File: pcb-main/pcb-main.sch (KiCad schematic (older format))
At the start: 26 parts, among them J1 AVR-ISP-6, J2 Conn_02x06_Counter_Clockwise, J3 Conn_02x02_Counter_Clockwise, M1 Stepper_Motor, U1 ATmega328P-AU, U2 HT1621B, U3 VIM878, U4 TLSM, Y1 Crystal

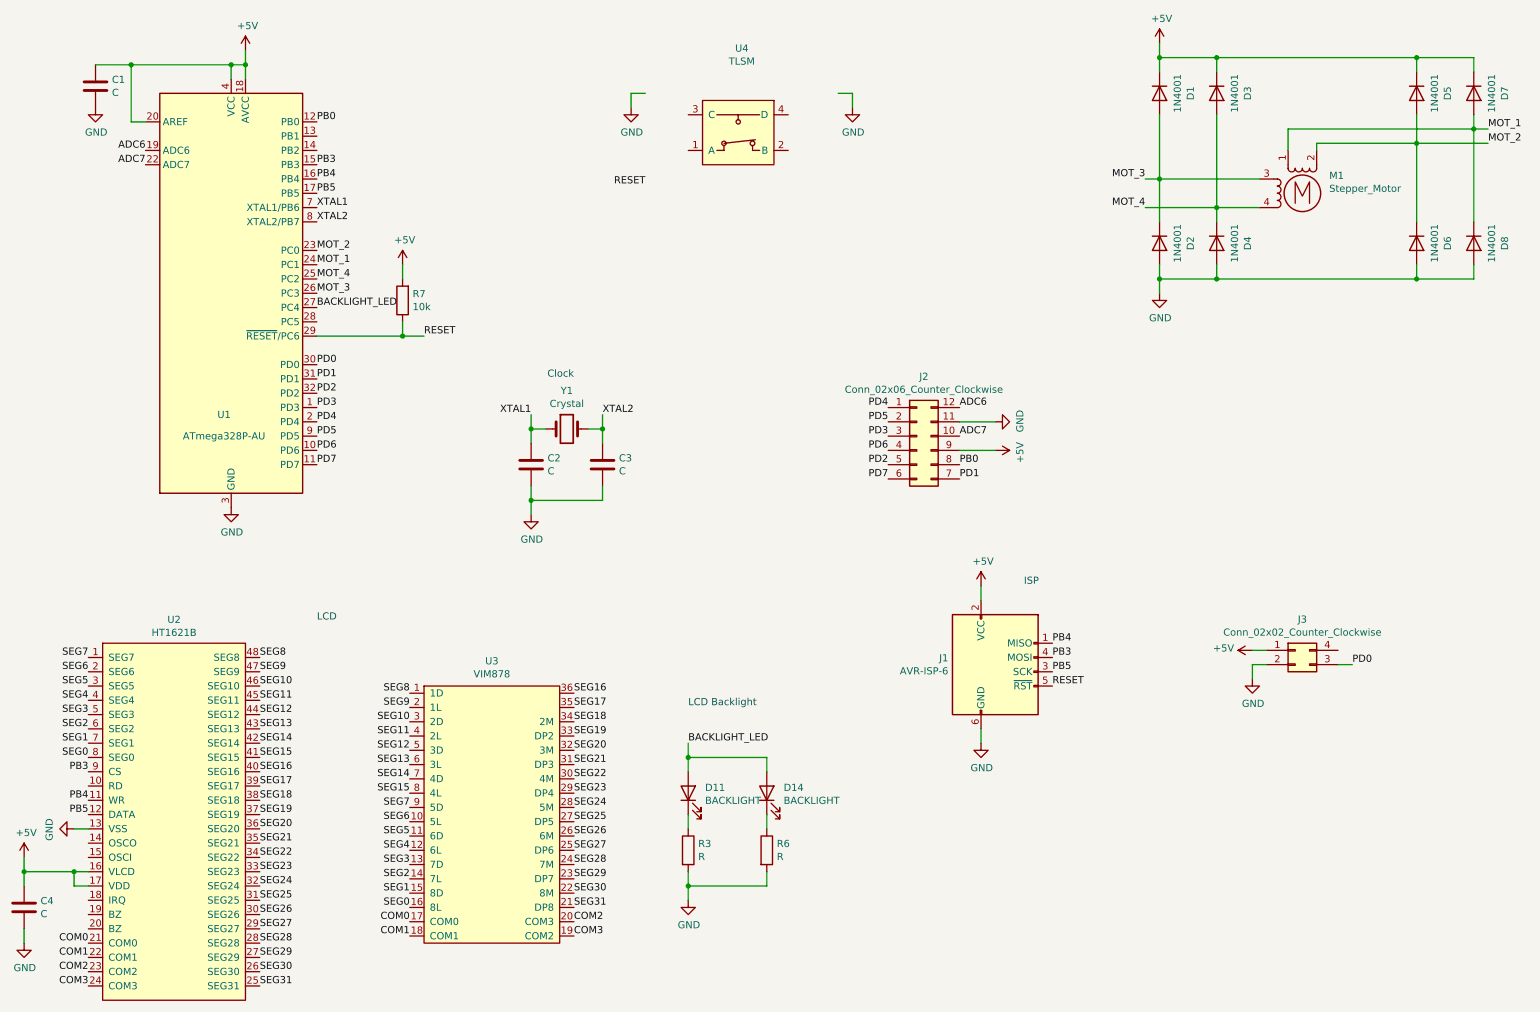
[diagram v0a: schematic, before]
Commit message: cleaned up main pcb
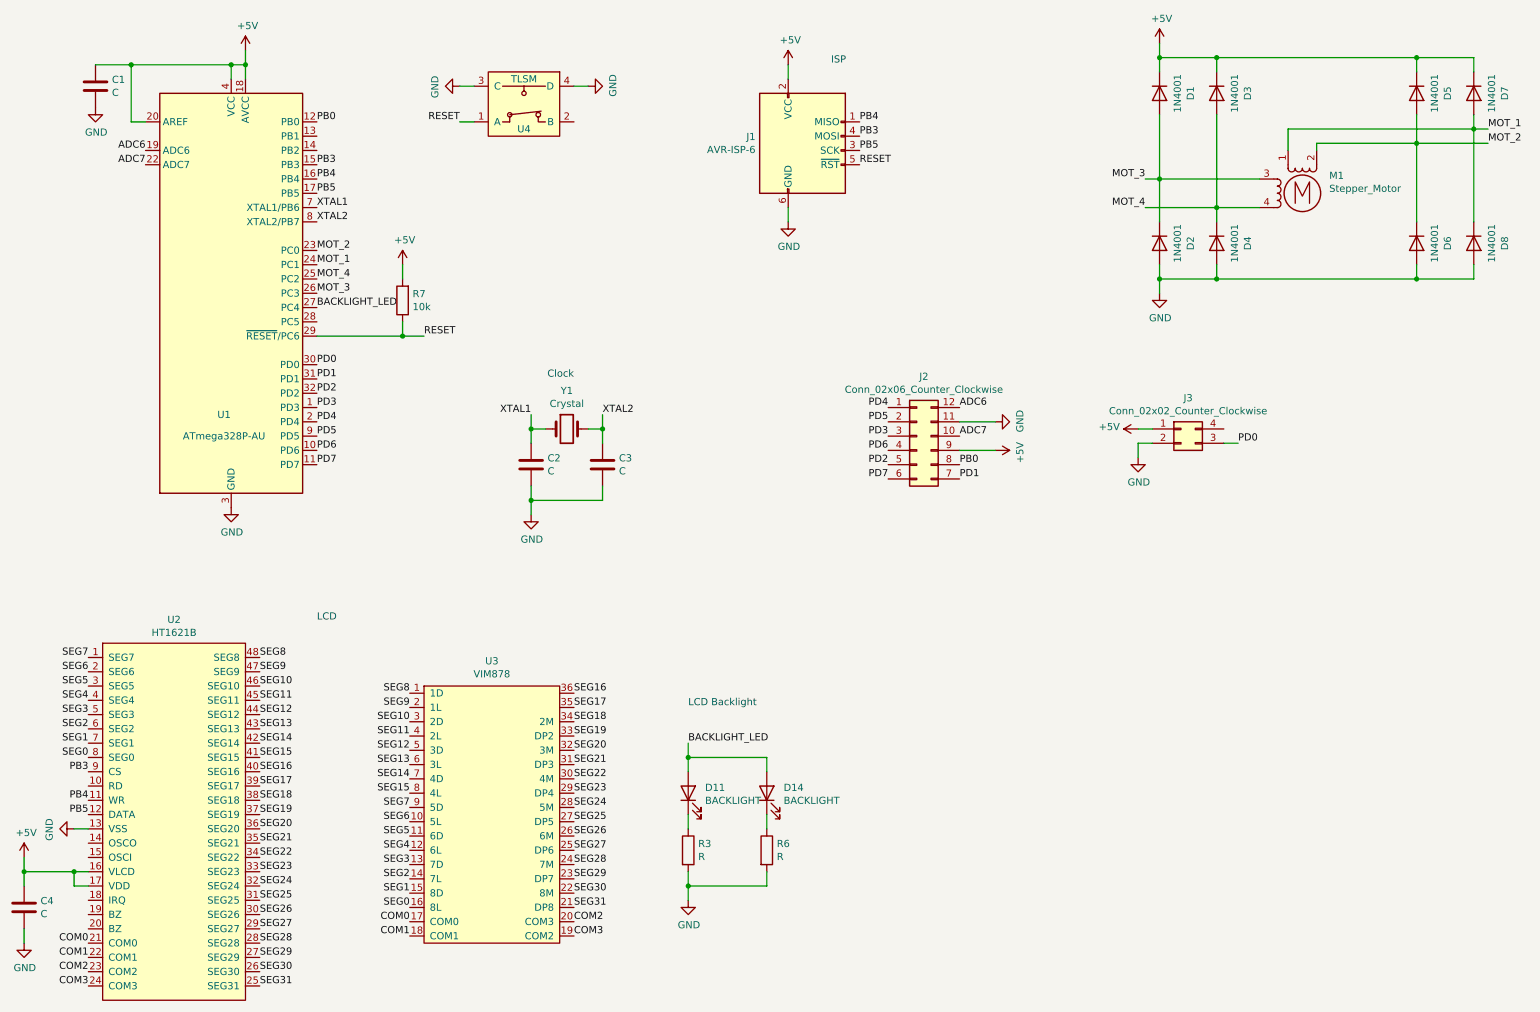
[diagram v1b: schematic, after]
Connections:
- net GND: now also U4.3 (C), U4.4 (D)
- net RESET: now also U4.1 (A)
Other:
- moved on the sheet: J1, J3, U4
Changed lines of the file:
@@
 L power:+5V #PWR?
 U 1 1 612E399D
-P 7300 4650
+P 5950 1000
 AR Path="/612034A3/612E399D" Ref="#PWR?"  Part="1"
 AR Path="/612E399D" Ref="#PWR0104"  Part="1"
-F 0 "#PWR0104" H 7300 4500 50  0001 C CNN
-F 1 "+5V" H 7315 4823 50  0000 C CNN
-F 2 "" H 7300 4650 50  0001 C CNN
-F 3 "" H 7300 4650 50  0001 C CNN
-	1    7300 4650
+F 0 "#PWR0104" H 5950 850 50  0001 C CNN
+F 1 "+5V" H 5965 1173 50  0000 C CNN
+F 2 "" H 5950 1000 50  0001 C CNN
+F 3 "" H 5950 1000 50  0001 C CNN
+	1    5950 1000
 	1    0    0    -1
 $EndComp
@@
 L power:GND #PWR?
 U 1 1 612E39A4
-P 7300 5750
+P 5950 2100
 AR Path="/612034A3/612E39A4" Ref="#PWR?"  Part="1"
 AR Path="/612E39A4" Ref="#PWR0105"  Part="1"
-F 0 "#PWR0105" H 7300 5500 50  0001 C CNN
-F 1 "GND" H 7305 5577 50  0000 C CNN
-F 2 "" H 7300 5750 50  0001 C CNN
-F 3 "" H 7300 5750 50  0001 C CNN
-	1    7300 5750
+F 0 "#PWR0105" H 5950 1850 50  0001 C CNN
+F 1 "GND" H 5955 1927 50  0000 C CNN
+F 2 "" H 5950 2100 50  0001 C CNN
+F 3 "" H 5950 2100 50  0001 C CNN
+	1    5950 2100
 	1    0    0    -1
 $EndComp
@@
 L Connector:AVR-ISP-6 J?
 U 1 1 612E39AB
-P 7400 5250
+P 6050 1600
 AR Path="/612034A3/612E39AB" Ref="J?"  Part="1"
 AR Path="/612E39AB" Ref="J1"  Part="1"
-F 0 "J1" H 7071 5346 50  0000 R CNN
-F 1 "AVR-ISP-6" H 7071 5255 50  0000 R CNN
-F 2 "Connector_PinHeader_2.54mm:PinHeader_2x03_P2.54mm_Vertical" V 7150 5300 50  0001 C CNN
-F 3 " ~" H 6125 4700 50  0001 C CNN
-	1    7400 5250
-	1    0    0    -1
-$EndComp
-Text Label 7800 5150 0    50   ~ 0
+F 0 "J1" H 5721 1696 50  0000 R CNN
+F 1 "AVR-ISP-6" H 5721 1605 50  0000 R CNN
+F 2 "Connector_PinHeader_2.54mm:PinHeader_2x03_P2.54mm_Vertical" V 5800 1650 50  0001 C CNN
+F 3 " ~" H 4775 1050 50  0001 C CNN
+	1    6050 1600
+	1    0    0    -1
+$EndComp
+Text Label 6450 1500 0    50   ~ 0
 PB3
-Text Label 7800 5050 0    50   ~ 0
+Text Label 6450 1400 0    50   ~ 0
 PB4
-Text Label 7800 5250 0    50   ~ 0
+Text Label 6450 1600 0    50   ~ 0
 PB5
-Text Label 7800 5350 0    50   ~ 0
+Text Label 6450 1700 0    50   ~ 0
 RESET
 Text Label 3400 2900 0    50   ~ 0
@@
 Connection ~ 2150 1000
 Wire Wire Line
-	7300 4650 7300 4750
-Wire Wire Line
-	7300 5650 7300 5750
+	5950 1000 5950 1100
+Wire Wire Line
+	5950 2000 5950 2100
 $Comp
 L Device:LED D11
@@
 Text Notes 2650 4900 0    50   ~ 0
 LCD
-Text Notes 7600 4650 0    50   ~ 0
+Text Notes 6250 1000 0    50   ~ 0
 ISP
 Wire Wire Line
@@
 L Connector_Generic:Conn_02x02_Counter_Clockwise J3
 U 1 1 61409762
-P 9500 5100
-F 0 "J3" H 9550 5317 50  0000 C CNN
-F 1 "Conn_02x02_Counter_Clockwise" H 9550 5226 50  0000 C CNN
-F 2 "Connector_PinHeader_2.54mm:PinHeader_2x02_P2.54mm_Vertical_SMD" H 9500 5100 50  0001 C CNN
-F 3 "~" H 9500 5100 50  0001 C CNN
-	1    9500 5100
+P 8700 3550
+F 0 "J3" H 8750 3767 50  0000 C CNN
+F 1 "Conn_02x02_Counter_Clockwise" H 8750 3676 50  0000 C CNN
+F 2 "Connector_PinHeader_2.54mm:PinHeader_2x02_P2.54mm_Vertical_SMD" H 8700 3550 50  0001 C CNN
+F 3 "~" H 8700 3550 50  0001 C CNN
+	1    8700 3550
 	1    0    0    -1
 $EndComp
 Text Label 2650 3100 0    50   ~ 0
 PD0
-Text Label 9900 5200 0    50   ~ 0
+Text Label 9100 3650 0    50   ~ 0
 PD0
 $Comp
 L power:+5V #PWR0112
 U 1 1 6140FFCF
-P 9200 5100
-F 0 "#PWR0112" H 9200 4950 50  0001 C CNN
-F 1 "+5V" V 9215 5228 50  0000 L CNN
-F 2 "" H 9200 5100 50  0001 C CNN
-F 3 "" H 9200 5100 50  0001 C CNN
-	1    9200 5100
+P 8400 3550
+F 0 "#PWR0112" H 8400 3400 50  0001 C CNN
+F 1 "+5V" V 8415 3678 50  0000 L CNN
+F 2 "" H 8400 3550 50  0001 C CNN
+F 3 "" H 8400 3550 50  0001 C CNN
+	1    8400 3550
 	0    -1   -1   0
 $EndComp
@@
 L power:GND #PWR0113
 U 1 1 614106F8
-P 9200 5300
-F 0 "#PWR0113" H 9200 5050 50  0001 C CNN
-F 1 "GND" H 9205 5127 50  0000 C CNN
-F 2 "" H 9200 5300 50  0001 C CNN
-F 3 "" H 9200 5300 50  0001 C CNN
-	1    9200 5300
-	1    0    0    -1
-$EndComp
-Wire Wire Line
-	9900 5200 9800 5200
-Wire Wire Line
-	9300 5100 9200 5100
-Wire Wire Line
-	9200 5300 9200 5200
-Wire Wire Line
-	9200 5200 9300 5200
+P 8400 3750
+F 0 "#PWR0113" H 8400 3500 50  0001 C CNN
+F 1 "GND" H 8405 3577 50  0000 C CNN
+F 2 "" H 8400 3750 50  0001 C CNN
+F 3 "" H 8400 3750 50  0001 C CNN
+	1    8400 3750
+	1    0    0    -1
+$EndComp
+Wire Wire Line
+	9100 3650 9000 3650
+Wire Wire Line
+	8500 3550 8400 3550
+Wire Wire Line
+	8400 3750 8400 3650
+Wire Wire Line
+	8400 3650 8500 3650
 $Comp
 L symbols:TLSM U4
 U 1 1 61493463
-P 5600 1500
-F 0 "U4" H 5625 2115 50  0000 C CNN
-F 1 "TLSM" H 5625 2024 50  0000 C CNN
-F 2 "footprints:TLSM" H 5600 1500 50  0001 C CNN
-F 3 "" H 5600 1500 50  0001 C CNN
-	1    5600 1500
-	1    0    0    -1
-$EndComp
-Text Label 4950 1850 2    50   ~ 0
+P 4100 1300
+F 0 "U4" H 4100 1150 50  0000 C CNN
+F 1 "TLSM" H 4100 1500 50  0000 C CNN
+F 2 "footprints:TLSM" H 4100 1300 50  0001 C CNN
+F 3 "" H 4100 1300 50  0001 C CNN
+	1    4100 1300
+	1    0    0    -1
+$EndComp
+Text Label 3650 1400 2    50   ~ 0
 RESET
 $Comp
 L power:GND #PWR0118
 U 1 1 6149B54A
-P 6400 1300
-F 0 "#PWR0118" H 6400 1050 50  0001 C CNN
-F 1 "GND" H 6405 1127 50  0000 C CNN
-F 2 "" H 6400 1300 50  0001 C CNN
-F 3 "" H 6400 1300 50  0001 C CNN
-	1    6400 1300
-	1    0    0    -1
-$EndComp
-Wire Wire Line
-	6300 1200 6400 1200
-Wire Wire Line
-	6400 1200 6400 1300
+P 4550 1150
+F 0 "#PWR0118" H 4550 900 50  0001 C CNN
+F 1 "GND" H 4555 977 50  0000 C CNN
+F 2 "" H 4550 1150 50  0001 C CNN
+F 3 "" H 4550 1150 50  0001 C CNN
+	1    4550 1150
+	0    -1   -1   0
+$EndComp
 $Comp
 L power:GND #PWR0119
 U 1 1 6149DF29
-P 4850 1300
-F 0 "#PWR0119" H 4850 1050 50  0001 C CNN
-F 1 "GND" H 4855 1127 50  0000 C CNN
-F 2 "" H 4850 1300 50  0001 C CNN
-F 3 "" H 4850 1300 50  0001 C CNN
-	1    4850 1300
-	1    0    0    -1
-$EndComp
-Wire Wire Line
-	4850 1300 4850 1200
-Wire Wire Line
-	4850 1200 4950 1200
+P 3650 1150
+F 0 "#PWR0119" H 3650 900 50  0001 C CNN
+F 1 "GND" H 3655 977 50  0000 C CNN
+F 2 "" H 3650 1150 50  0001 C CNN
+F 3 "" H 3650 1150 50  0001 C CNN
+	1    3650 1150
+	0    1    1    0
+$EndComp
+Wire Wire Line
+	3750 1400 3650 1400
+Wire Wire Line
+	3650 1150 3750 1150
+Wire Wire Line
+	4450 1150 4550 1150
 $EndSCHEMATC
